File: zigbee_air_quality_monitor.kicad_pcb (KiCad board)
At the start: 4 copper layers, 41 parts, among them J1 USB_C_Receptacle_USB2.0, J2 QWIIC, J3 Conn_02x02_Odd_Even, SW1 PAIR_BTN, SW2 USER_BTN, U1 USBLC6-2SC6, U2 BT840, U3 XC6206P332MR, U4 SCD41-D-R2

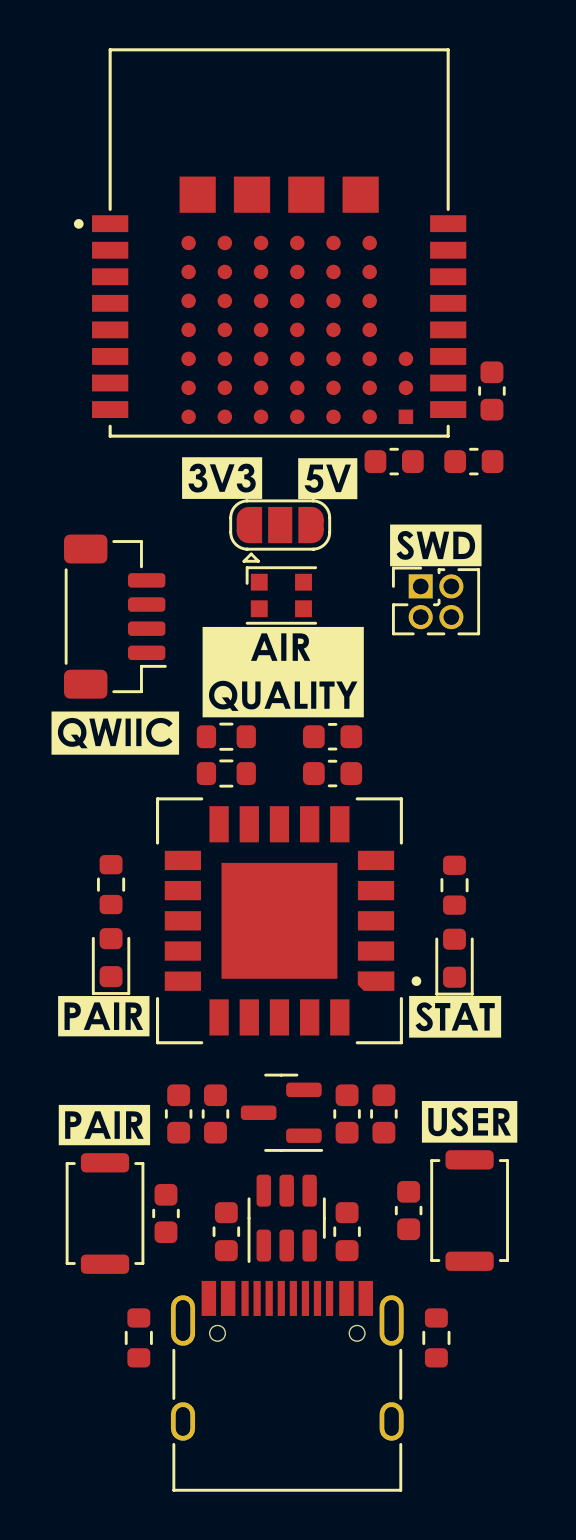
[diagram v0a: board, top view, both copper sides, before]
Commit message: Routing WIP
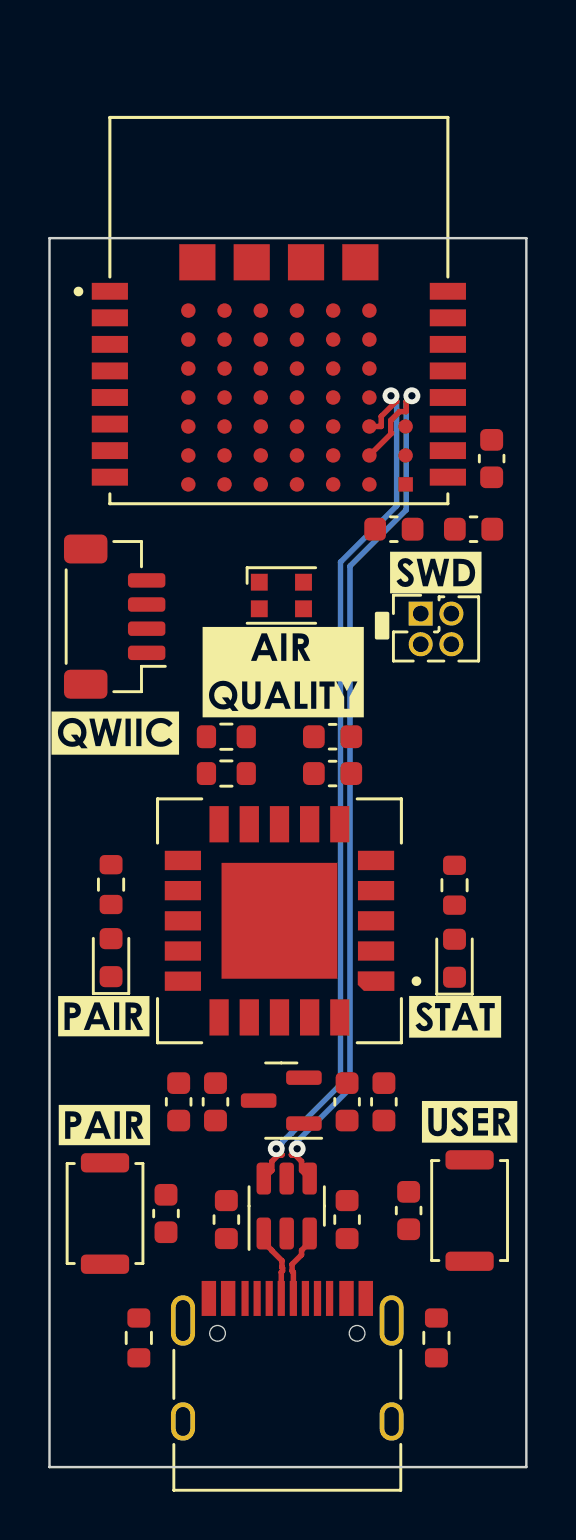
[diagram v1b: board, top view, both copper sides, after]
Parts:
- removed JP1: SolderJumper_3_Bridged12, Jumper:SolderJumper-3_P1.3mm_Open_RoundedPad1.0x1.5mm
- removed kibuzzard-63D645FF: G***, kibuzzard-63D645FF
- removed kibuzzard-63D6461A: G***, kibuzzard-63D6461A
- moved C3 2.80 mm to (136.4, 101.3)
- moved C4 2.80 mm to (140.4, 98.3)
- moved C6 2.80 mm to (139.7, 101.3)
- moved U2 2.80 mm to (131.6, 92.2)
- moved J3 1.12 mm to (137.5, 104.8)
- moved kibuzzard-63D64107 1.12 mm to (138.1, 103.0)
- moved U3 0.50 mm to (131.7, 124.9)
- moved C5 0.50 mm to (127.5, 125.0)
- moved C7 0.50 mm to (129.0, 125.0)
- moved C8 0.50 mm to (134.4, 125.0)
- moved C9 0.50 mm to (135.9, 125.0)
- moved F1 0.50 mm to (129.4, 129.8)
- moved FB1 0.50 mm to (134.4, 129.8)
- moved U1 0.50 mm to (131.9, 129.3)
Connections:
- D3 pad 1: Net-(D3-Pad1) -> +3.3V
- J1 pad A6: /USB_CONN_D- -> /USB_CONN_D+
- J1 pad A7: /USB_CONN_D+ -> /USB_CONN_D-
- J1 pad B6: /USB_CONN_D- -> /USB_CONN_D+
- J1 pad B7: /USB_CONN_D+ -> /USB_CONN_D-
- U1 pad 1: /USB_CONN_D- -> /USB_CONN_D+
- U1 pad 3: /USB_CONN_D+ -> /USB_CONN_D-
- U1 pad 4: /USB_D+ -> /USB_D-
- U1 pad 6: /USB_D- -> /USB_D+
- U2 pad 13: unconnected-(U2-Pad13) -> /STATUS_LED
- U2 pad 14: unconnected-(U2-Pad14) -> /PAIRING_LED
- U2 pad 7: /STATUS_LED -> unconnected-(U2-P0.09/NFC1-Pad7)
- U2 pad 8: /PAIRING_LED -> unconnected-(U2-P0.10/NFC2-Pad8)
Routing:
- net /USB_D-: track 0.00 -> 38.3 mm, vias 0 -> 2
- net /USB_D+: track 0.00 -> 37.2 mm, vias 0 -> 2
- net /USB_CONN_D+: track 0.00 -> 3.03 mm
- net /USB_CONN_D-: track 0.00 -> 3.01 mm
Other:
- board outline added: 19.8 x 50.9 mm
